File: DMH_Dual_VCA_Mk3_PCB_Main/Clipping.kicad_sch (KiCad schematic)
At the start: 48 parts, among them Q10 BC548, Q11 BC548, Q12 BC548, Q9 BC548, SW2 SW_DPDT_OnOffOn_x2, U10 TL074

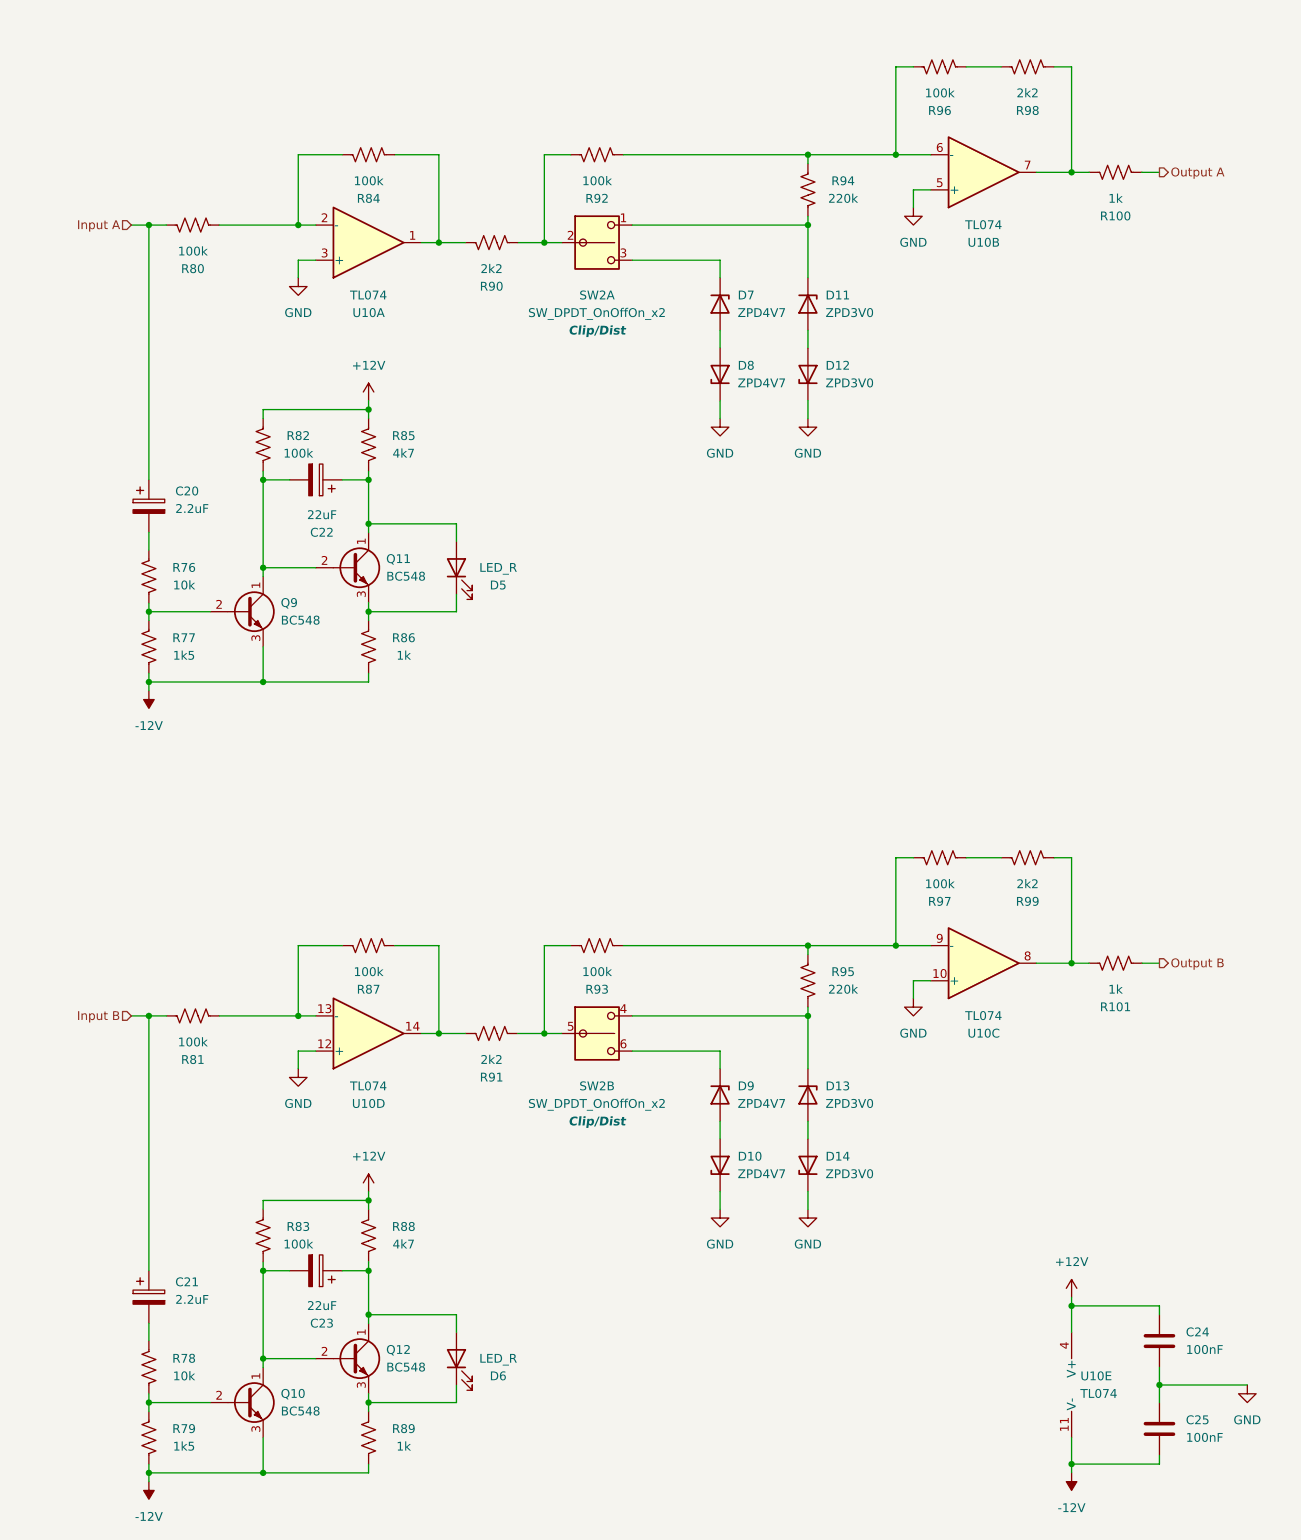
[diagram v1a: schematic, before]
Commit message: Started Main PCB comp placement
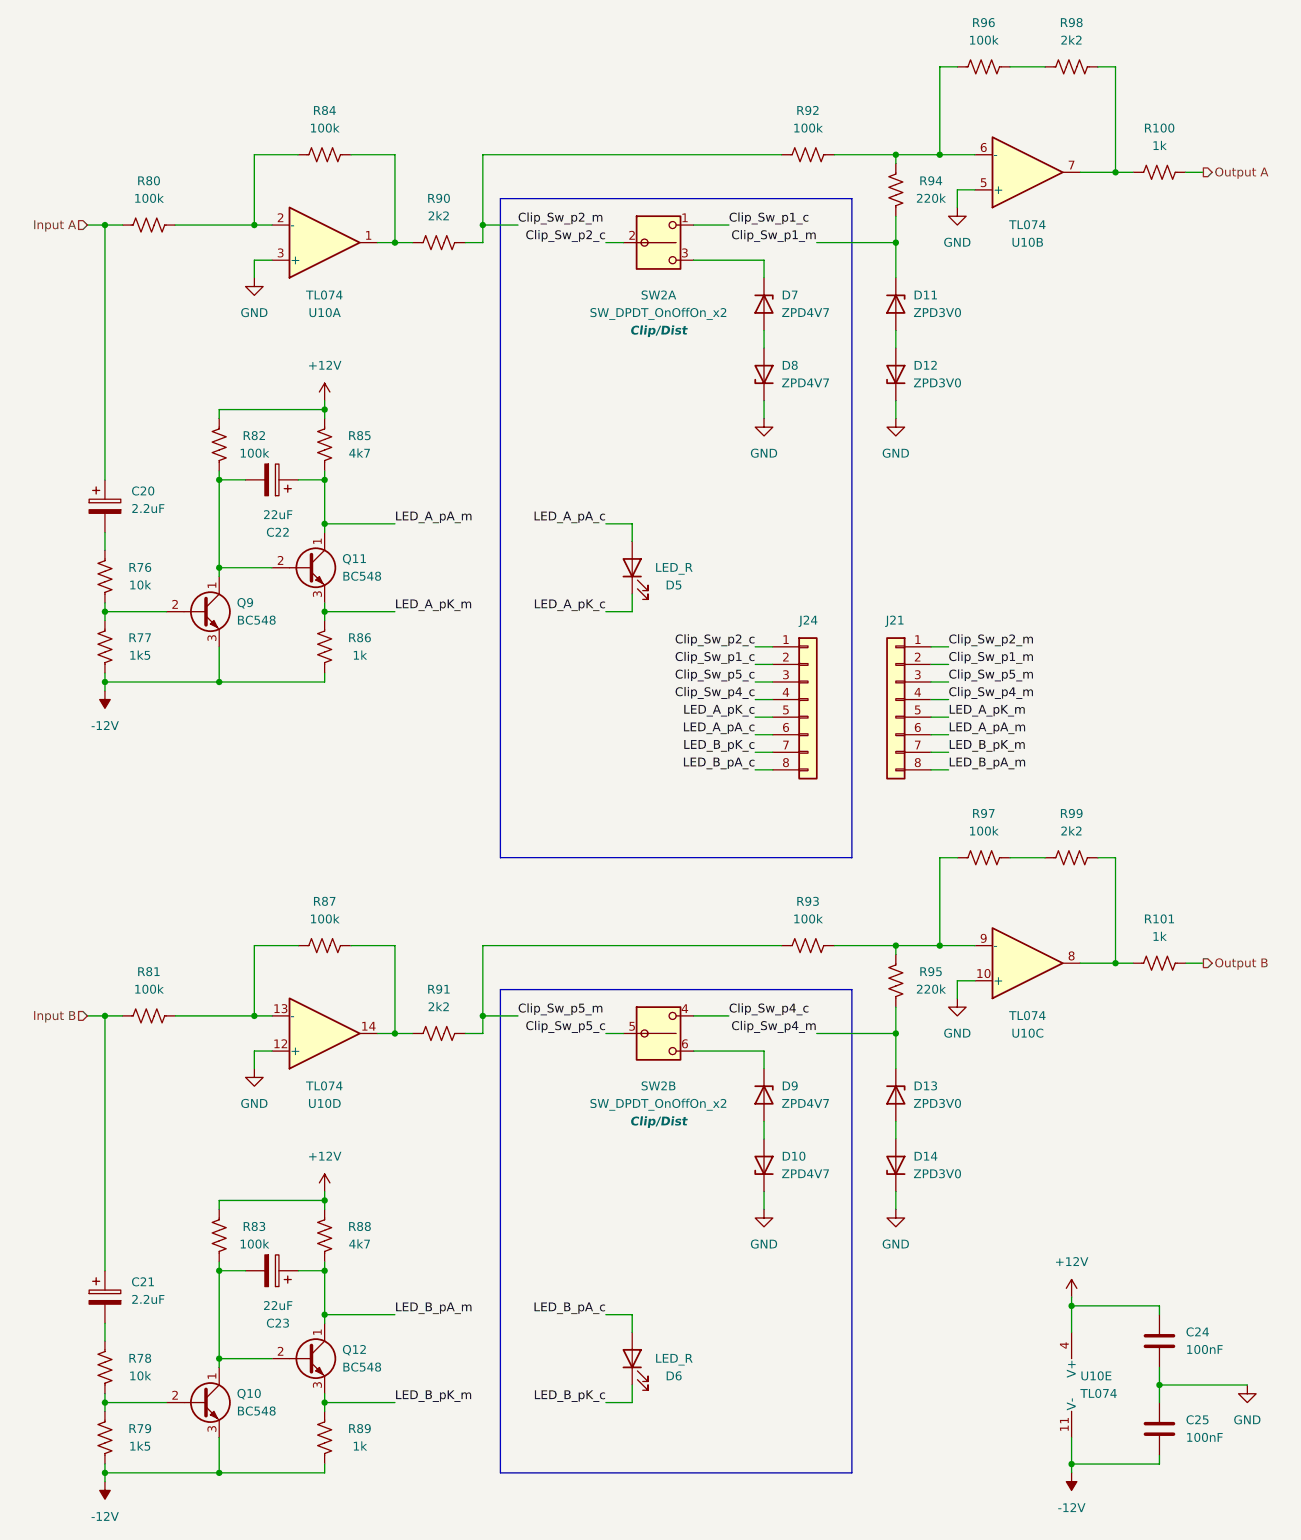
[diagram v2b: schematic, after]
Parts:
- added J21: Conn_01x08, Connector_PinHeader_2.54mm:PinHeader_1x08_P2.54mm_Vertical, symbol Connector_Generic:Conn_01x08
- added J24: Conn_01x08, Connector_PinSocket_2.54mm:PinSocket_1x08_P2.54mm_Vertical, symbol Connector_Generic:Conn_01x08
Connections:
- net Clip_Sw_p5_m: now reaches R91.2, R93.1
- net Clip_Sw_p5_m: now also J21.3 (Pin_3); no longer SW2.5 (B)
- net LED_A_pA_m: now reaches C22.1, Q11.1 (C), R85.1
- net LED_A_pA_m: now also J21.6 (Pin_6); no longer D5.2 (A)
- net LED_B_pK_m: now reaches Q12.3 (E), R89.2
- net LED_B_pK_m: now also J21.7 (Pin_7); no longer D6.1 (K)
- net Clip_Sw_p2_m: now reaches R90.2, R92.1
- net Clip_Sw_p2_m: now also J21.1 (Pin_1); no longer SW2.2 (B)
- net LED_B_pA_m: now reaches C23.1, Q12.1 (C), R88.1
- net LED_B_pA_m: now also J21.8 (Pin_8); no longer D6.2 (A)
- net LED_A_pK_m: now reaches Q11.3 (E), R86.2
- net LED_A_pK_m: now also J21.5 (Pin_5); no longer D5.1 (K)
- net Clip_Sw_p1_m: now reaches D11.1 (K), R94.1
- net Clip_Sw_p1_m: now also J21.2 (Pin_2); no longer SW2.1 (A)
- net Clip_Sw_p4_m: now reaches D13.1 (K), R95.1
- net Clip_Sw_p4_m: now also J21.4 (Pin_4); no longer SW2.4 (A)
- new net Clip_Sw_p1_c: J24.2 (Pin_2), SW2.1 (A)
- new net Clip_Sw_p2_c: J24.1 (Pin_1), SW2.2 (B)
- new net Clip_Sw_p4_c: J24.4 (Pin_4), SW2.4 (A)
- new net Clip_Sw_p5_c: J24.3 (Pin_3), SW2.5 (B)
- new net LED_A_pA_c: D5.2 (A), J24.6 (Pin_6)
- new net LED_A_pK_c: D5.1 (K), J24.5 (Pin_5)
- new net LED_B_pA_c: D6.2 (A), J24.8 (Pin_8)
- new net LED_B_pK_c: D6.1 (K), J24.7 (Pin_7)
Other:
- moved on the sheet: C20, C21, C22, C23, D10, D11, D12, D13, D14, D5, D6, D7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

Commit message: Main comp placement in progress
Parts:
- Q10, Q11, Q12, Q9: footprint Package_TO_SOT_THT:TO-92_Inline -> Package_TO_SOT_THT:TO-92L_Inline_Wide
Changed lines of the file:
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@@
 			)
 		)
-		(property "Footprint" "Package_TO_SOT_THT:TO-92_Inline"
+		(property "Footprint" "Package_TO_SOT_THT:TO-92L_Inline_Wide"
 			(at 59.69 226.695 0)
 			(hide yes)
@@
 			)
 		)
-		(property "Footprint" "Package_TO_SOT_THT:TO-92_Inline"
+		(property "Footprint" "Package_TO_SOT_THT:TO-92L_Inline_Wide"
 			(at 59.69 112.395 0)
 			(hide yes)
@@
 			)
 		)
-		(property "Footprint" "Package_TO_SOT_THT:TO-92_Inline"
+		(property "Footprint" "Package_TO_SOT_THT:TO-92L_Inline_Wide"
 			(at 44.45 118.745 0)
 			(hide yes)
@@
 			)
 		)
-		(property "Footprint" "Package_TO_SOT_THT:TO-92_Inline"
+		(property "Footprint" "Package_TO_SOT_THT:TO-92L_Inline_Wide"
 			(at 44.45 233.045 0)
 			(hide yes)
